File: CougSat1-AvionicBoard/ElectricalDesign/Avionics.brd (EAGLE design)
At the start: 90.4 x 95.8 mm, 219 parts, among them J1 +X Panel GPS, J10 iFJR SD1, J11 -Y, J12 +Z, J13 +X, J14 -Z, J15 +Y, J16 IFJR SD0, J2 IHU SD1, J3 SWD, J4 CougSat Card, J5 -X, J6 IHU SD0, J8 SWD, J9 SWD, U1 STM32L476RGT, U10 BNO055, U11 M24M01, U12 TXS0102DQM, U13 TXS0102DQM, U14 AD8515, U15 BNO055, U16 BNO055, U17 TXS0102DQM, U18 TXS0102DQM, U19 AD8515, U2 STM32L476RGT, U20 INA199C2, U21 INA199C2, U22 TXS0102DQM, U23 TXS0102DQM, U24 AD8515, U25 AD7291, U26 AD7291, U27 TXS0102DQM, U28 INA199C2, U29 AD8515, U3 STM32L476RGT, U30 DRV8837, U4 M24M01, U5 TXS0102DQM, U6 DRV8837, U7 DRV8837, U8 AD7291, U9 Venus838FLPx-L, Y1 8MHz ±10ppm, Y10 32.768kHz ±10ppm, Y2 32.768kHz ±10ppm, Y3 8MHz ±10ppm, Y4 32.768kHz ±10ppm, Y5 8MHz ±10ppm, Y6 32.768kHz ±10ppm, Y7 32.768kHz ±10ppm, Y8 32.768kHz ±10ppm

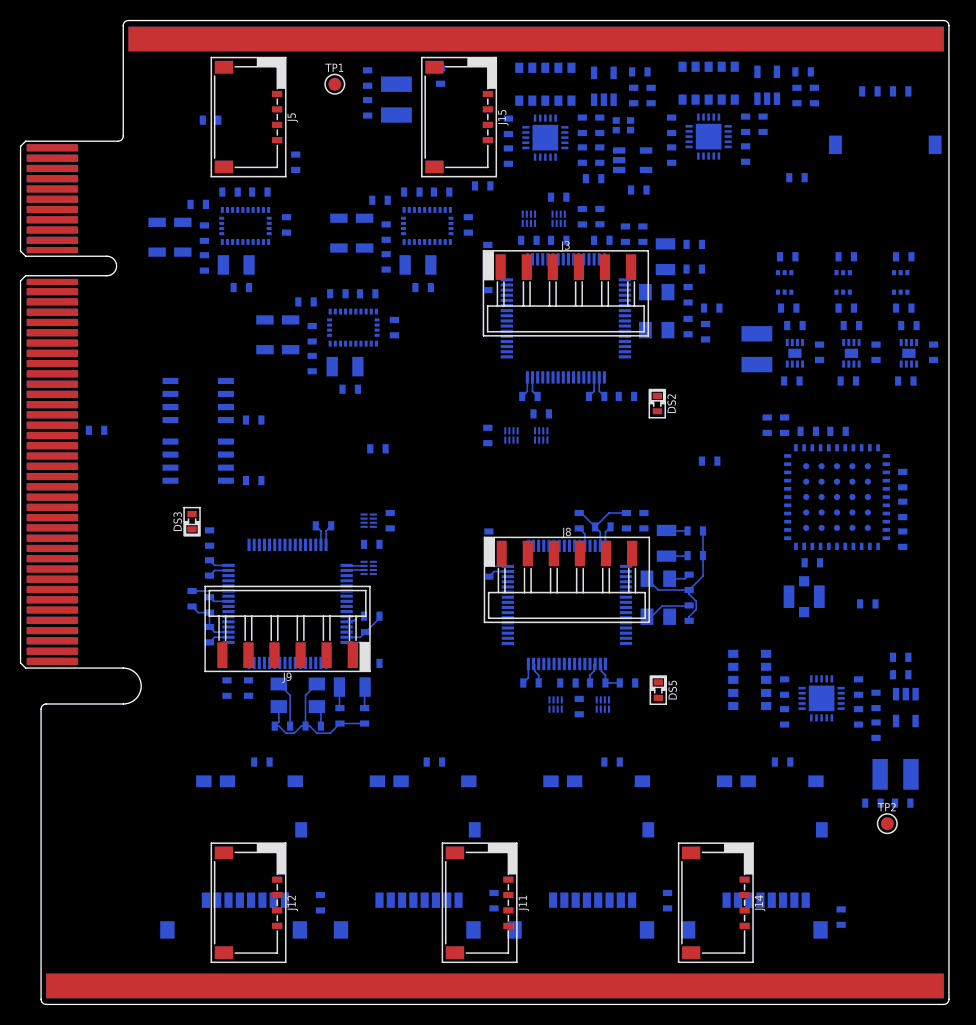
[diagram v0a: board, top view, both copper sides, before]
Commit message: Routed Most Traces
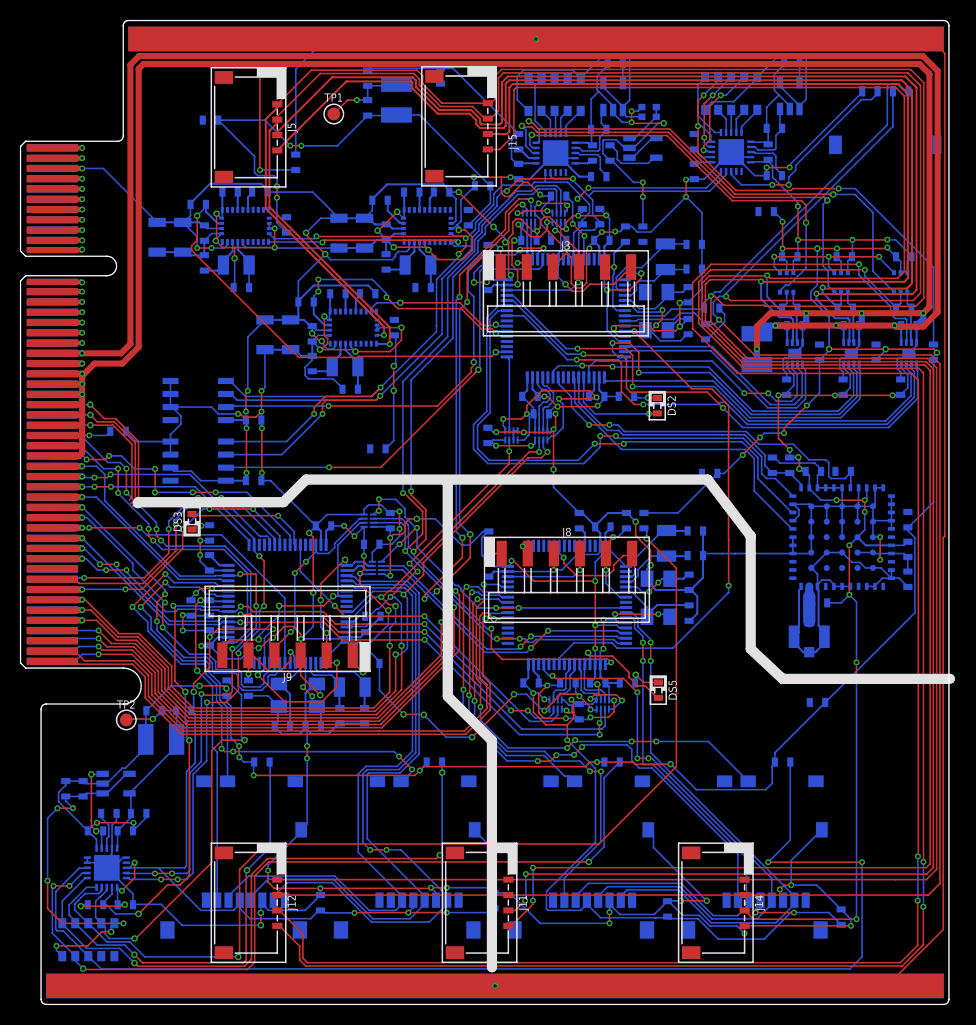
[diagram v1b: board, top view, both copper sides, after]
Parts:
- removed C44, C51, C67: 1µF 10%, CougsInSpace-Capacitors:1608
- removed C50, C52, C68: 100nF 10%, CougsInSpace-Capacitors:1608
- moved C70 82.3 mm to (4.40, -26.9), turned to 90 degrees
- moved C69 80.4 mm to (6.10, -26.9), turned to 90 degrees
- moved U29 77.3 mm to (9.30, -26.4), turned to 180 degrees
- moved C64 75.6 mm to (7.30, -31.0), turned to 0 degrees
- moved C88 75.5 mm to (8.60, -29.3), turned to 180 degrees
- moved TP2 74.8 mm to (10.3, -20.2)
- moved C94 73.5 mm to (13.0, -19.3), turned to 0 degrees
- moved C65 72.3 mm to (10.2, -31.0), turned to 180 degrees
- moved C84 72.3 mm to (11.5, -29.3), turned to 180 degrees
- moved C93 71.6 mm to (13.7, -22.1), turned to 180 degrees
- moved U26 71.5 mm to (8.40, -34.6), turned to 180 degrees
- moved R7 70.4 mm to (7.30, -38.2), turned to 0 degrees
- moved RN3 69.2 mm to (6.60, -41.6), turned to 0 degrees
- moved FB2 67.7 mm to (15.9, -19.3), turned to 0 degrees
- moved C15 66.8 mm to (10.2, -38.2), turned to 180 degrees
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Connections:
- removed net COIL-X_OUT1: R29.1, U20.4, U30.2
- removed net COIL-Y_OUT1: R30.1, U21.4, U6.2
- removed net COIL-Z_OUT1: R31.1, U28.4, U7.2
- new net COIL-X_OUT2: R29.1, U20.4, U30.3
- new net COIL-Y_OUT2: R30.1, U21.4, U6.3
- new net COIL-Z_OUT2: R31.1, U28.4, U7.3
- net ADCS_ADC0_VREF: no longer RN1.3
- net ADCS_HALF_REF: no longer C44.1, C50.1
- net AGND: no longer C44.2, C50.2, C51.2, C52.2, C67.2, C68.2
- net AVREF-0: now also RN1.3; no longer C51.1, C52.1
- net AVREF-1: no longer C67.1, C68.1
- net COIL-X_!SLEEP: now also U2.27; no longer U2.20
- net COIL-X_COIL+: now also U30.2; no longer R29.2, U20.5
- net COIL-X_COIL-: now also R29.2, U20.5; no longer U30.3
- net COIL-X_IN1: now also U2.16; no longer U2.14
- net COIL-X_IN2: now also U2.17; no longer U2.15
- net COIL-Y_!SLEEP: now also U2.20; no longer U2.27
- net COIL-Y_COIL+: now also U6.2; no longer R30.2, U21.5
- net COIL-Y_COIL-: now also R30.2, U21.5; no longer U6.3
- net COIL-Y_IN1: now also U2.14; no longer U2.16
- net COIL-Y_IN2: now also U2.15; no longer U2.17
- net COIL-Z_COIL+: now also U7.2; no longer R31.2, U28.5
- net COIL-Z_COIL-: now also R31.2, U28.5; no longer U7.3
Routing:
- net DGND: track 61.0 -> 713.3 mm, vias 0 -> 85
- net 3.3V_2: track 4.11 -> 381.3 mm, vias 0 -> 43
- net AGND: track 0.00 -> 338.0 mm, vias 0 -> 33
- net ADCS_I2C1_SCL: track 0.00 -> 319.8 mm, vias 0 -> 2
- net ADCS_I2C1_SDA: track 0.00 -> 318.1 mm, vias 0 -> 3
- net PGND: track 0.00 -> 238.6 mm, vias 0 -> 9
- net COIL-Y_COIL+: track 0.00 -> 212.6 mm, vias 0 -> 3
- net COIL-Y_COIL-: track 0.00 -> 210.8 mm, vias 0 -> 3
- net CHASSIS: track 0.00 -> 204.6 mm, vias 0 -> 2
- net 3.3V_0: track 11.6 -> 189.5 mm, vias 0 -> 29
- net COIL-Z_COIL+: track 0.00 -> 177.2 mm, vias 0 -> 3
- net COIL-Z_COIL-: track 0.00 -> 173.1 mm, vias 0 -> 3
- net VBATT_5: track 0.00 -> 167.2 mm, vias 0 -> 4
- net 3.3V_5: track 8.23 -> 155.5 mm, vias 0 -> 20
- net BUS_JTAG_TMS: track 0.00 -> 132.1 mm, vias 0 -> 6
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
